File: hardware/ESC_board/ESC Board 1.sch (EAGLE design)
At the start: 15 parts

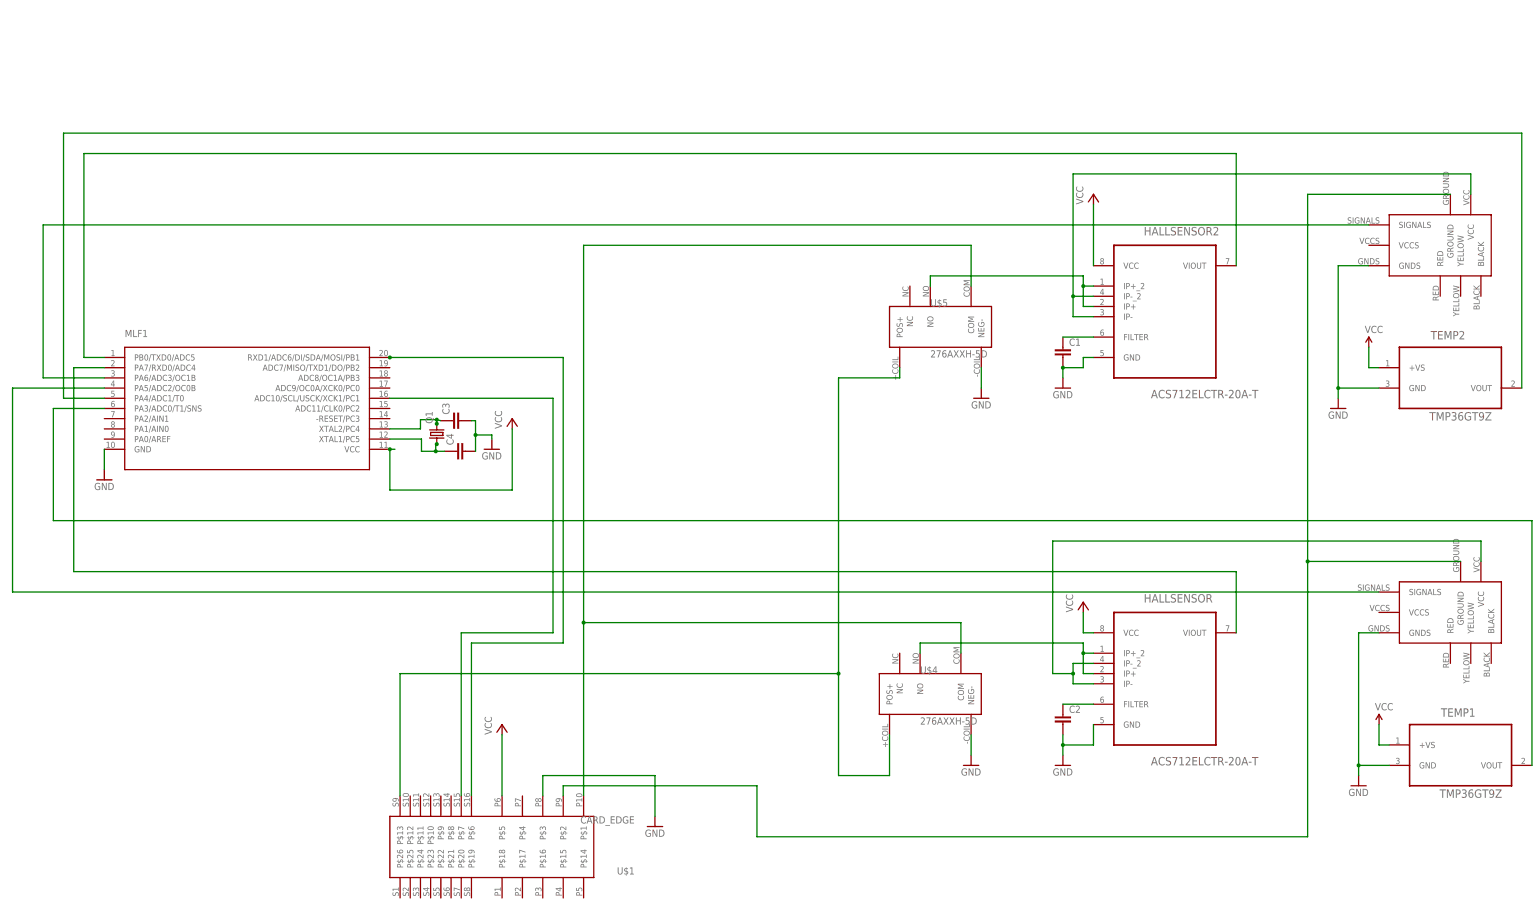
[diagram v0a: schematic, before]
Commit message: total redesign is way better
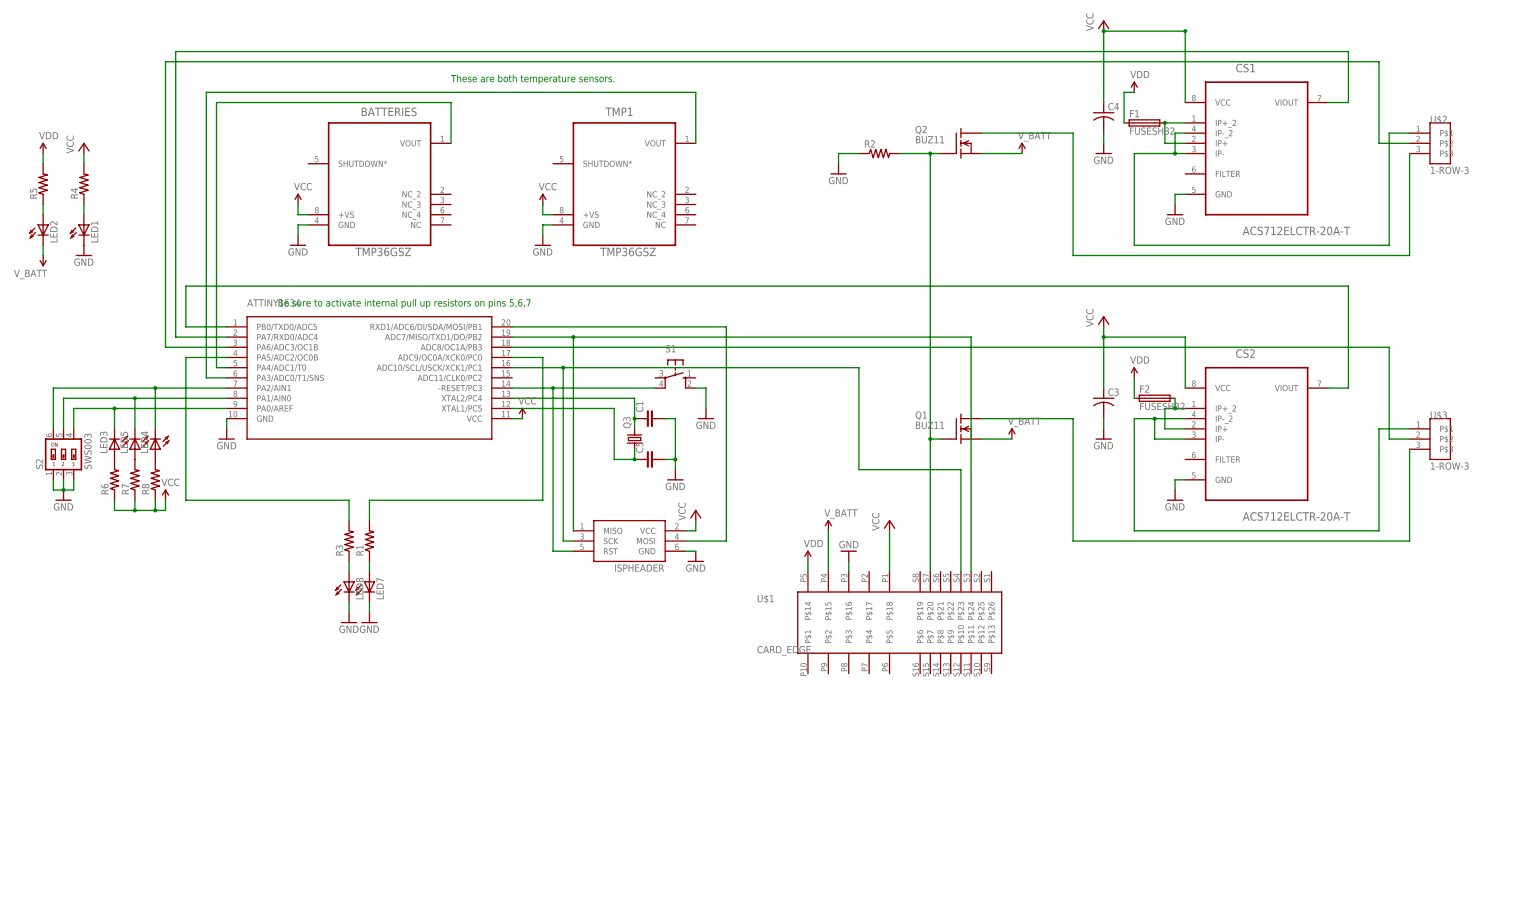
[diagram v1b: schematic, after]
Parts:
- removed C2: (no value), SparkFun-Capacitors:CAPEZ
- removed HALLSENSOR, HALLSENSOR2: ACS712ELCTR-20A-T, Allegro_By_element14_Batch_1:ACS712ELCTR-20A-T
- removed MLF1: ATTINY1634SOIC20, attiny1634:ATTINY1634SOIC20
- removed TEMP1, TEMP2: TMP36GT9Z, ADI-Phase-2:TMP36GT9Z
- removed U$4, U$5: 276AXXH-5D, Schneider Relay:276AXXH-5D
- added ATTINY1634: ATTINY1634SOIC20, attiny1634:ATTINY1634SOIC20
- added BATTERIES, TMP1: TMP36GSZ, ADI-Phase-2:TMP36GSZ
- added C5: (no value), SparkFun-Capacitors:0.1UF-50V-20%(PTH)KIT-EZ
- added CS1, CS2: ACS712ELCTR-20A-T, Allegro_By_element14_Batch_1:ACS712ELCTR-20A-T
- added F1, F2: FUSESH32, fuse:FUSESH32
- added ISPHEADER: AVRISP-6, adafruit:AVRISP-6
- added LED1, LED2, LED3, LED4, LED5, LED7, LED8: (no value), adafruit:LEDCHIP-LED0805
- added Q2: BUZ11, transistor-fet:BUZ11
- added Q3: (no value), crystal:CRYSTALHC49S
- added R1, R2, R3, R4, R5, R6, R7, R8: (no value), adafruit:R-US_M2012
- added S1: (no value), switch-omron:10-XX
- added S2: SWS003, smd-special:SWS003
- C1: device SparkFun-Capacitors:CAPEZ -> SparkFun-Capacitors:0.1UF-50V-20%(PTH)KIT-EZ
- C3, C4: device SparkFun-Capacitors:CAPEZ -> rcl:C-US025-030X050
- Q1: value (none) -> BUZ11; device crystal:CRYTALTC26V -> transistor-fet:BUZ11
- U$2, U$3: value ESC30A -> 1-ROW-3; device ESC-30A:ESC30A -> con-molex-mini-fit:1-ROW-3
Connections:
- removed net BAT-: U$1.P$2, U$2.GROUND, U$3.GROUND
- new net N$18: ATTINY1634.RXD1/ADC6/DI/SDA/MOSI/PB1, ISPHEADER.MOSI
- new net N$20: ATTINY1634.XTAL2/PC4, C1.1, Q3.2
- new net N$21: LED5.A, R7.2
- new net N$22: ATTINY1634.PA3/ADC0/T1/SNS, TMP1.VOUT
- new net N$23: LED4.A, R8.2
- new net N$24: ATTINY1634.PA6/ADC3/OC1B, U$2.P$2
- new net N$25: LED2.A, R5.1
- new net N$26: ATTINY1634.ADC8/OC1A/PB3, U$3.P$2
- new net N$27: LED8.A, R3.1
- new net N$28: LED7.A, R1.1
- new net N$32: LED1.A, R4.1
- new net N$35: CS1.IP+, CS1.IP+_2, F1.2
- new net N$36: CS2.IP+, CS2.IP+_2, F2.2
- new net VDD: F1.1, F2.1, R5.2, U$1.P$14
- new net V_BATT: LED2.C, Q1.S, Q2.S, U$1.P$15
- net GND: now also ATTINY1634.GND, BATTERIES.GND, C5.2, CS1.GND, CS2.GND, ISPHEADER.GND, LED1.C, LED7.C, LED8.C, R2.1, S1.S1, S2.1, S2.2, S2.3, TMP1.GND, U$1.P$16; no longer C2.2, HALLSENSOR.GND, HALLSENSOR2.GND, MLF1.GND, TEMP1.GND, TEMP2.GND, U$1.P$3, U$2.GNDS, U$3.GNDS, U$4.NEG-, U$5.NEG-
- net N$1: now also ATTINY1634.ADC9/OC0A/XCK0/PC0, R1.2; no longer MLF1.PA4/ADC1/T0, TEMP2.VOUT
- net N$10: now also ATTINY1634.PA4/ADC1/T0, BATTERIES.VOUT; no longer HALLSENSOR2.IP-, HALLSENSOR2.IP-_2, U$3.VCC
- net N$11: now also ATTINY1634.PA2/AIN1, LED4.C, S2.6; no longer U$1.P$1, U$4.COM, U$5.COM
- net N$12: now also ATTINY1634.PA1/AIN0, LED5.C, S2.5; no longer HALLSENSOR.IP-, HALLSENSOR.IP-_2, U$2.VCC
- net N$13: now also ATTINY1634.PA0/AREF, LED3.C, S2.4; no longer MLF1.PA5/ADC2/OC0B, U$2.SIGNALS
- net N$14: now also LED3.A, R6.2; no longer MLF1.PA6/ADC3/OC1B, U$3.SIGNALS
- net N$15: now also CS1.IP-, CS1.IP-_2, U$2.P$1; no longer C2.1, HALLSENSOR.FILTER
- net N$16: now also ATTINY1634.ADC10/SCL/USCK/XCK1/PC1, ISPHEADER.SCK, U$1.P$23; no longer HALLSENSOR.IP+, HALLSENSOR.IP+_2, U$4.NO
- net N$17: now also ATTINY1634.-RESET/PC3, ISPHEADER.RST, S1.P1; no longer HALLSENSOR2.IP+, HALLSENSOR2.IP+_2, U$5.NO
- net N$19: now also ATTINY1634.XTAL1/PC5, C5.1, Q3.1; no longer U$1.P$13, U$4.POS+, U$5.POS+
- net N$2: now also Q1.G, Q2.G, R2.2, U$1.P$20; no longer MLF1.PA3/ADC0/T1/SNS, TEMP1.VOUT
- net N$3: now also ATTINY1634.PA5/ADC2/OC0B, R3.2; no longer MLF1.RXD1/ADC6/DI/SDA/MOSI/PB1, U$1.P$6
- net N$4: now also Q1.D, U$3.P$3; no longer MLF1.ADC10/SCL/USCK/XCK1/PC1, U$1.P$7
- net N$5: now also Q2.D, U$2.P$3; no longer HALLSENSOR2.VIOUT, MLF1.PB0/TXD0/ADC5
- net N$6: now also ATTINY1634.ADC7/MISO/TXD1/DO/PB2, ISPHEADER.MISO, U$1.P$24; no longer HALLSENSOR.VIOUT, MLF1.PA7/RXD0/ADC4
- net N$7: now also CS2.IP-, CS2.IP-_2, U$3.P$1; no longer C3.1, MLF1.XTAL2/PC4, Q1.2
- net N$8: now also ATTINY1634.PB0/TXD0/ADC5, CS2.VIOUT; no longer C4.1, MLF1.XTAL1/PC5, Q1.1
- net N$9: now also ATTINY1634.PA7/RXD0/ADC4, CS1.VIOUT; no longer C1.1, HALLSENSOR2.FILTER
- net VCC: now also ATTINY1634.VCC, BATTERIES.+VS, C3.1, C4.1, CS1.VCC, CS2.VCC, ISPHEADER.VCC, R4.2, R6.1, R7.1, R8.1, TMP1.+VS, U$1.P$18; no longer HALLSENSOR.VCC, HALLSENSOR2.VCC, MLF1.VCC, TEMP1.+VS, TEMP2.+VS, U$1.P$5
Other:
- note added: "Be sure to activate internal pull up resistors on pins 5,6,7"
- note added: "These are both temperature sensors."
- moved on the sheet: C1, C3, C4, U$1
